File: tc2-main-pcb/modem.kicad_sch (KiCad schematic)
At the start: 29 parts, among them J111 Conn_01x08, J112 Screw_Terminal_01x01, U116 SIM7600G-H-M.2, U121 TPS62A02DRLR

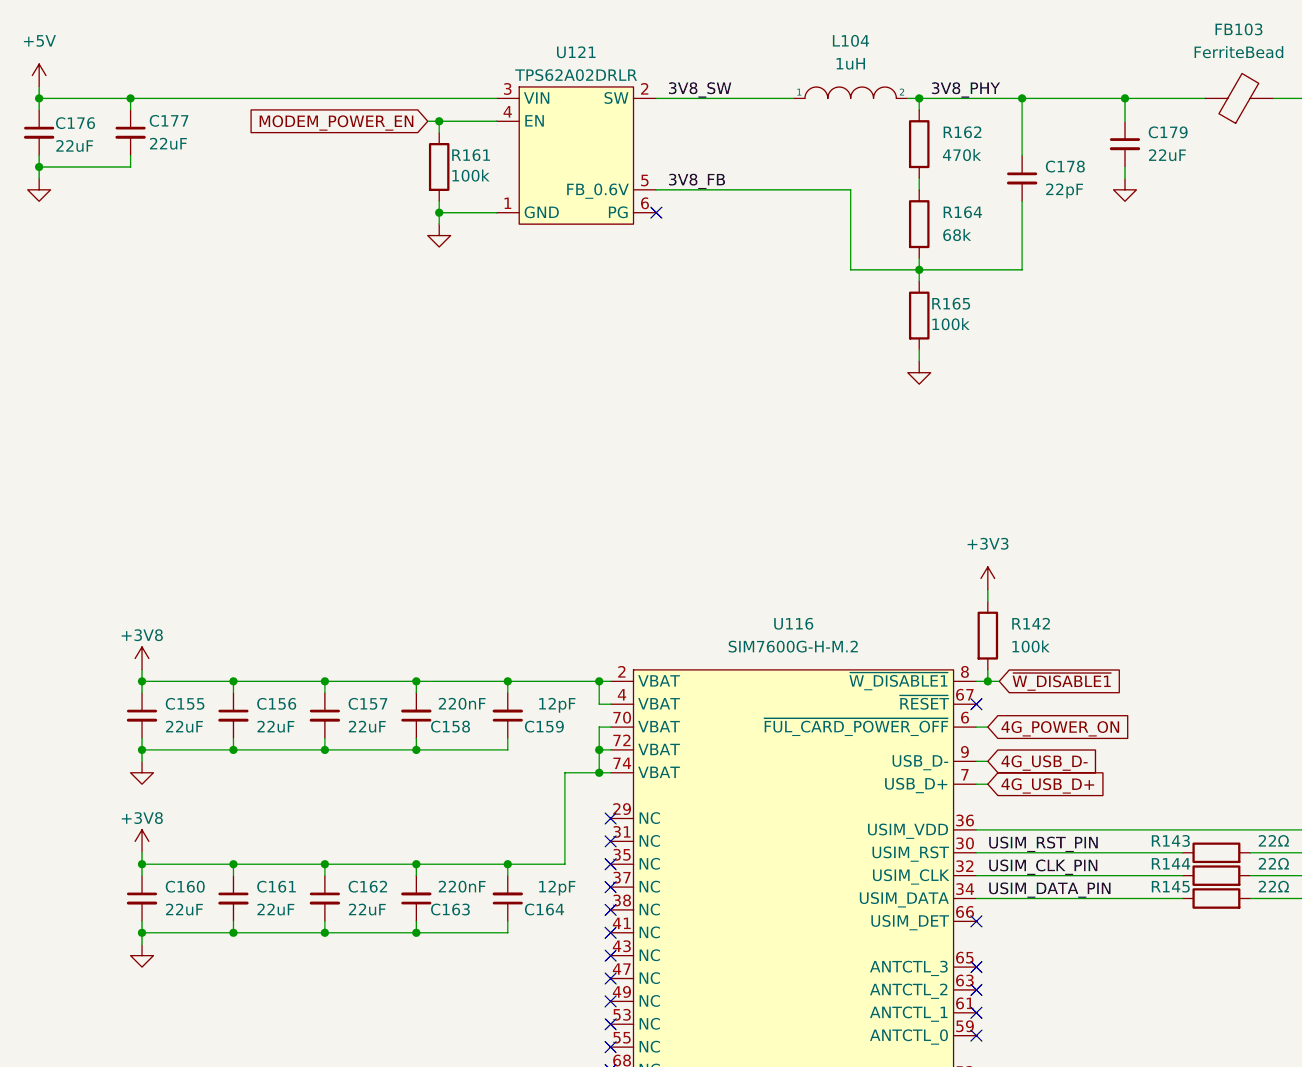
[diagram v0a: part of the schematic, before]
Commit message: Update schematic
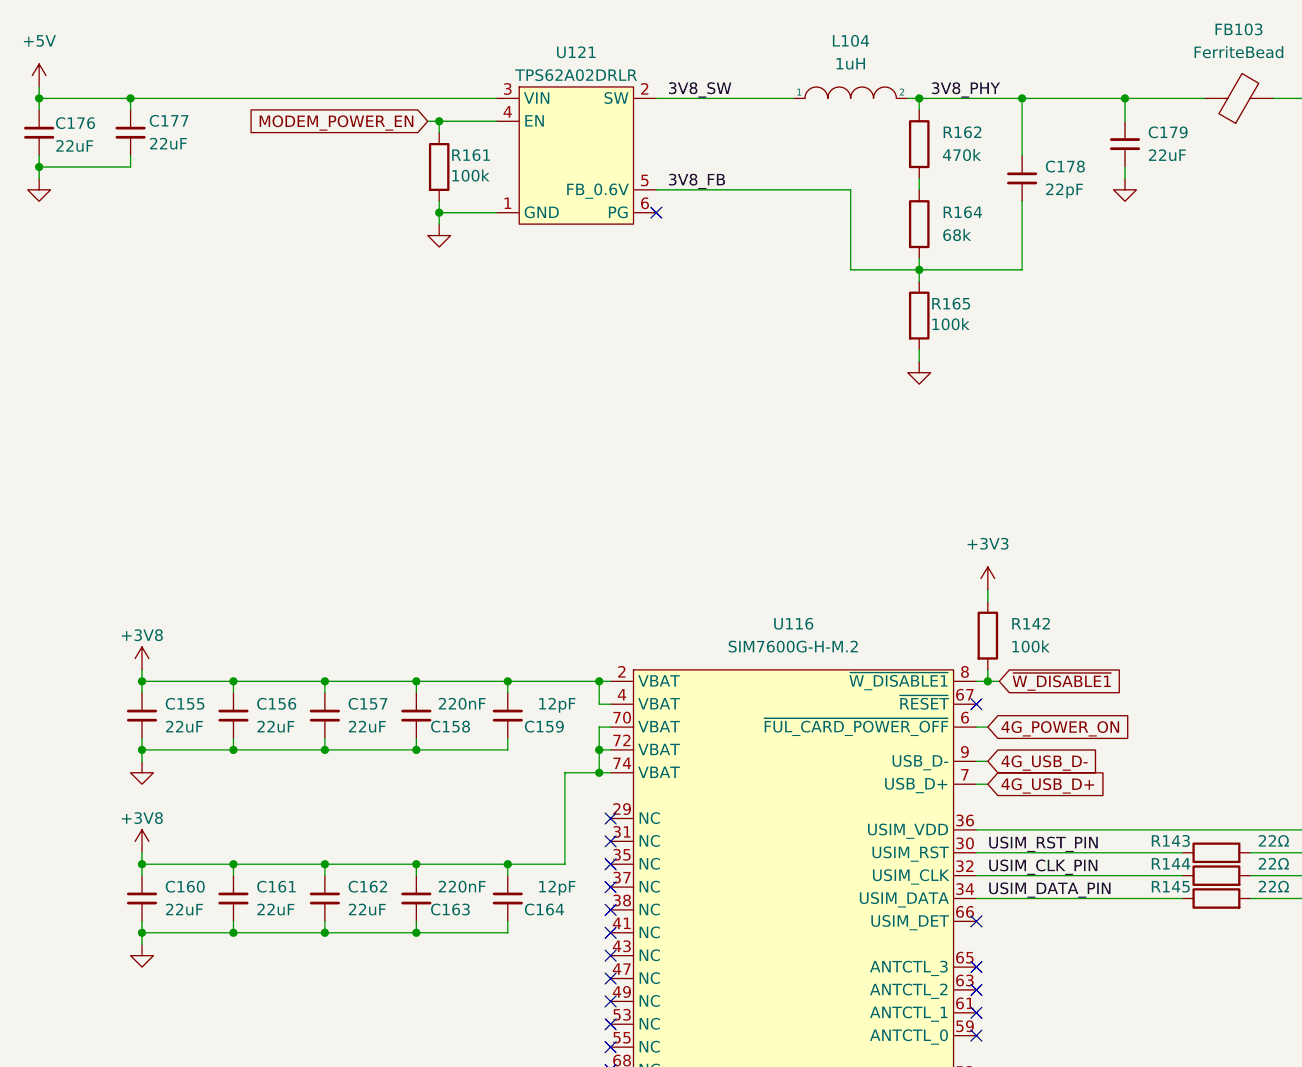
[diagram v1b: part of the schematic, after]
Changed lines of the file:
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@@
 			)
 		)
-		(property "Description" ""
+		(property "Description" "Unpolarized capacitor, small symbol"
 			(at 60.96 92.71 0)
 			(hide yes)
@@
 			)
 		)
-		(property "Description" ""
+		(property "Description" "Unpolarized capacitor, small symbol"
 			(at 40.64 113.03 0)
 			(hide yes)
